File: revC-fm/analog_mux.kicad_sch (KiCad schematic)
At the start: 33 parts, among them J2 T1M-08-F-SV-L, U10 OPA340MDBVTEP, U11 74HC4067PW,118

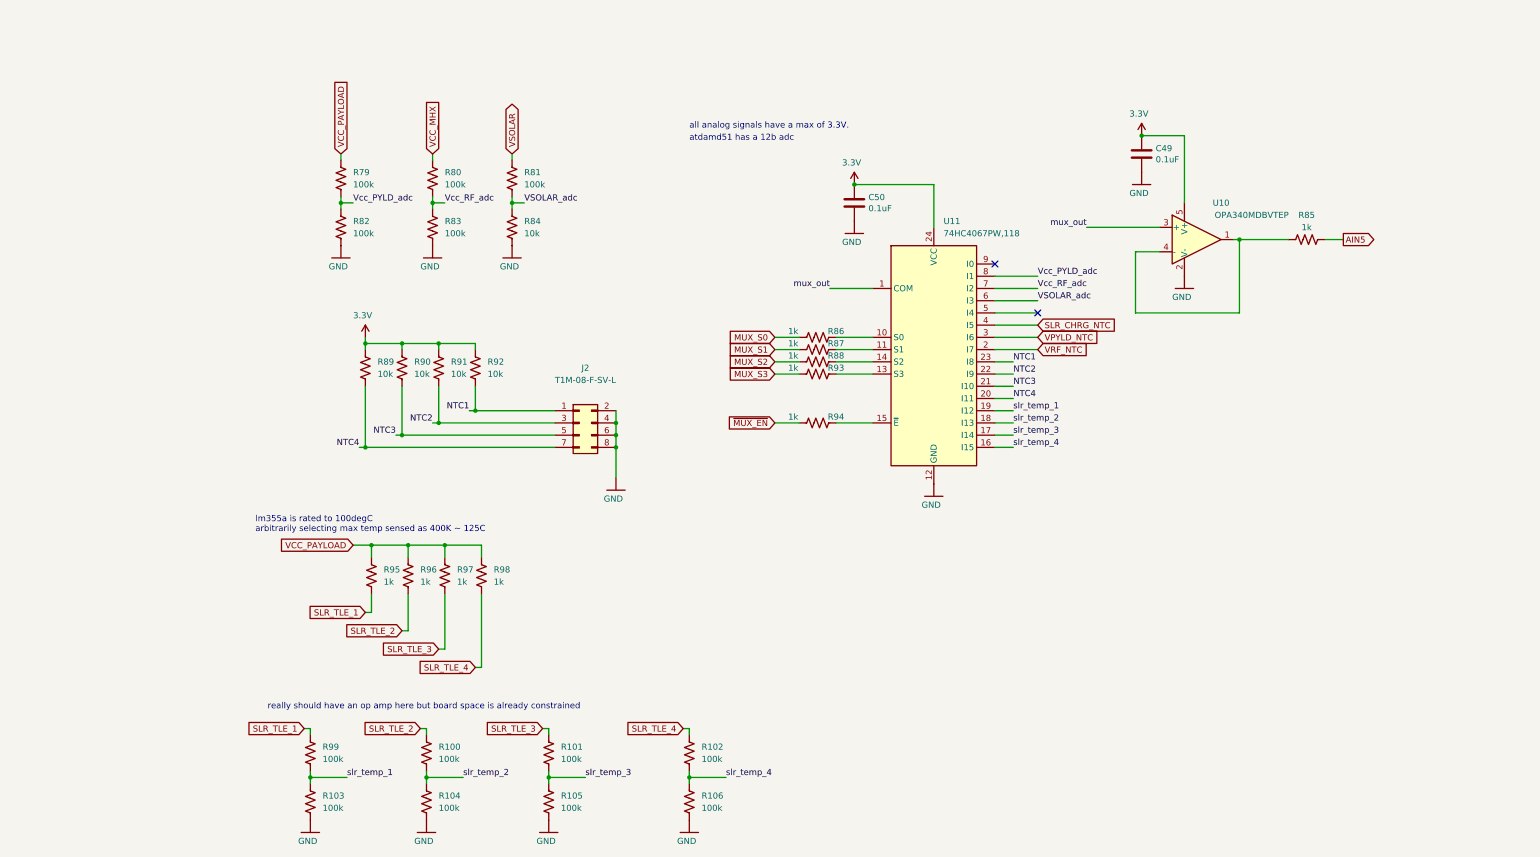
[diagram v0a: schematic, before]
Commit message: working revC
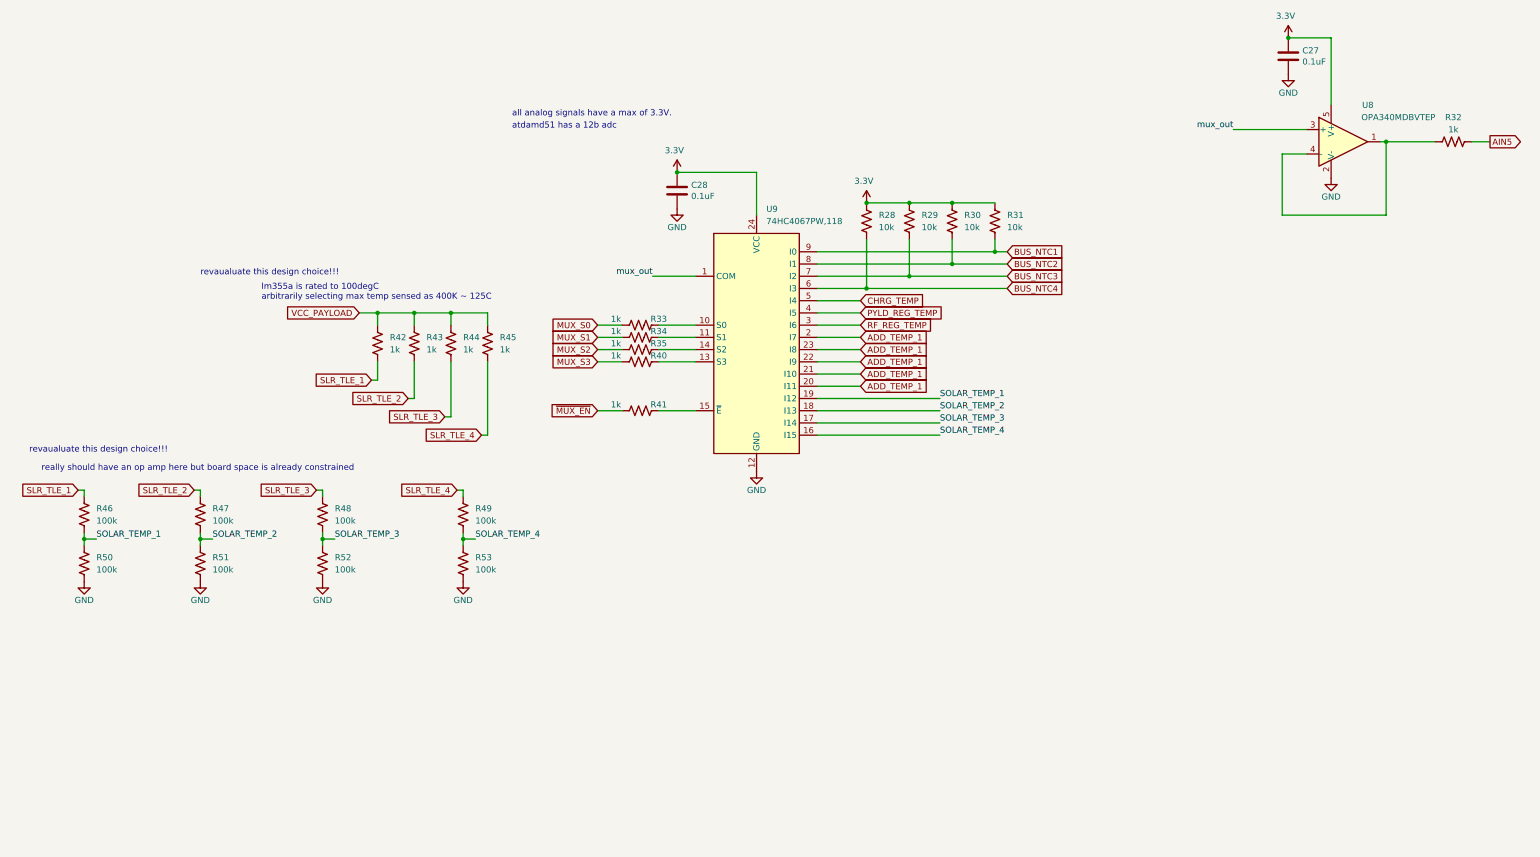
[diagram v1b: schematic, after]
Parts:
- removed J2: T1M-08-F-SV-L, mainboard-SLI:SAMTEC_T1M-08-F-SV-L, symbol Connector_Generic:Conn_02x04_Odd_Even
- removed R79, R80, R81, R82, R83: 100k, Resistor_SMD:R_0603_1608Metric, symbol Device:R_US
- removed R84, R89, R90, R91, R92: 10k, Resistor_SMD:R_0603_1608Metric, symbol Device:R_US
- added R28, R29, R30, R31: 10k, Resistor_SMD:R_0603_1608Metric, symbol Device:R_US
- renumbered C49 to C27, C50 to C28, R85 to R32, R86 to R33, R87 to R34, R88 to R35, R93 to R40, R94 to R41, R95 to R42, R96 to R43, R97 to R44, R98 to R45, R99 to R46, R100 to R47, R101 to R48, R102 to R49, R103 to R50, R104 to R51, R105 to R52, R106 to R53, U10 to U8, U11 to U9
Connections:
- net NTC2 is gone; now on net ADD_TEMP_1: U9.22 (I9)
- net NTC3 is gone; now on net ADD_TEMP_1: U9.21 (I10)
- net NTC4 is gone; now on net ADD_TEMP_1: U9.20 (I11)
- net VRF_NTC is gone; now on net ADD_TEMP_1: U9.2 (I7)
- net 3.3V: now also R28.1, R29.1, R30.1, R31.1
- net CHRG_TEMP: now reaches U9.5 (I4)
- net BUS_NTC1: now reaches U9.9 (I0)
- net BUS_NTC1: now also R31.2
- net NTC1 renamed ADD_TEMP_1
- net SLR_CHRG_NTC renamed PYLD_REG_TEMP
- net VPYLD_NTC renamed RF_REG_TEMP
- net VSOLAR_adc renamed BUS_NTC4
- net BUS_NTC4: now also R28.2
- net Vcc_PYLD_adc renamed BUS_NTC2
- net BUS_NTC2: now also R30.2
- net Vcc_RF_adc renamed BUS_NTC3
- net BUS_NTC3: now also R29.2
- net slr_temp_1 renamed SOLAR_TEMP_1
- net slr_temp_2 renamed SOLAR_TEMP_2
- net slr_temp_3 renamed SOLAR_TEMP_3
- net slr_temp_4 renamed SOLAR_TEMP_4
- no-connect marks 2 -> 0
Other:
- note added: "revaualuate this design choice!!!"
- moved on the sheet: C27, C28, R32, R33, R34, R35, R40, R41, R42, R43, R44, R45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
